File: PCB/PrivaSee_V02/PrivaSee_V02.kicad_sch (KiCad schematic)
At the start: 35 parts, among them J1 RFPC-SMA27-F, J2 Batt_Solder_Point, J3 Conn_02x06_Odd_Even, J4 VOUT_TEST, J5 GND_TEST, J6 IR_TEST, J7 RF_TEST, SW1 Switch, U1 RC1602A, U2 LM358, U3 254, U4 DFR0568, U6 ESP32-C5-DevKitC-1

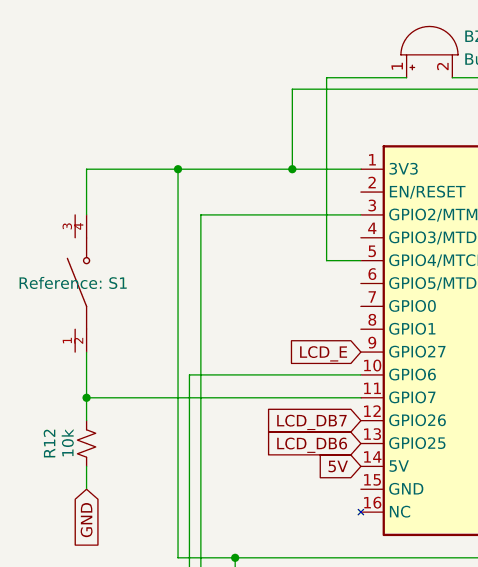
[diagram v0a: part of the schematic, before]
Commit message: button update
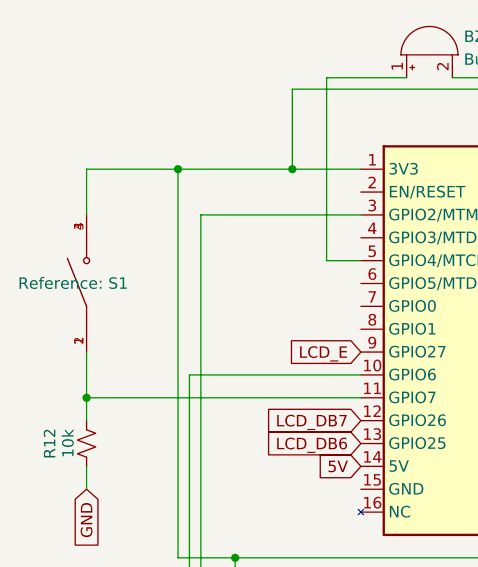
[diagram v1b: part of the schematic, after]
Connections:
- net 3V3: now also S1.3
- net at R12.2, S1.2, U6.11 (GPIO7): now also S1.1
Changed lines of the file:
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@@
+	(wire
+		(pts
+			(xy 34.29 57.15) (xy 34.29 62.23)
+		)
+		(stroke
+			(width 0)
+			(type default)
+		)
+	)
 	(wire
 		(pts
@@
 	(wire
 		(pts
+			(xy 34.29 77.47) (xy 34.29 82.55)
+		)
+		(stroke
+			(width 0)
+			(type default)
+		)
+	)
+	(wire
+		(pts
 			(xy 45.72 80.01) (xy 45.72 162.56)
 		)
@@
 	(wire
 		(pts
-			(xy 34.29 57.15) (xy 34.29 62.23)
-		)
-		(stroke
-			(width 0)
-			(type default)
-		)
-	)
-	(wire
-		(pts
 			(xy 46.99 62.23) (xy 64.77 62.23)
 		)
@@
 		)
 		(stroke
-			(width 0)
-			(type default)
-		)
-	)
-	(wire
-		(pts
-			(xy 34.29 77.47) (xy 34.29 82.55)
-		)
-		(stroke
